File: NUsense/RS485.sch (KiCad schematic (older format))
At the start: 7 parts, among them J1101 MOLEX22-03-5045, U1101 MAX3443ECSA+

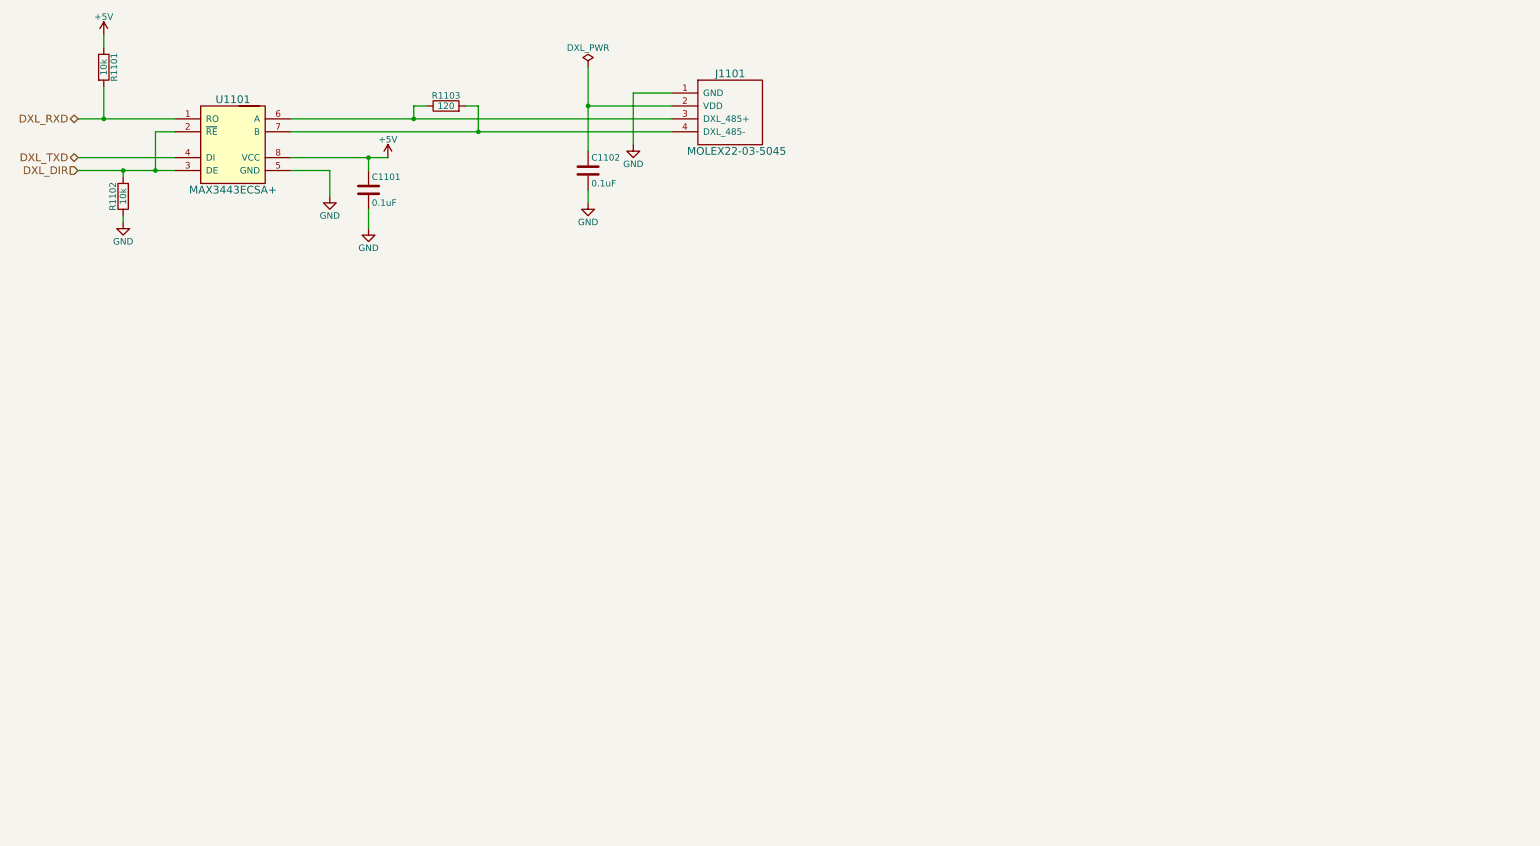
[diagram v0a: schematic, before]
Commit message: Cleans up some minor things
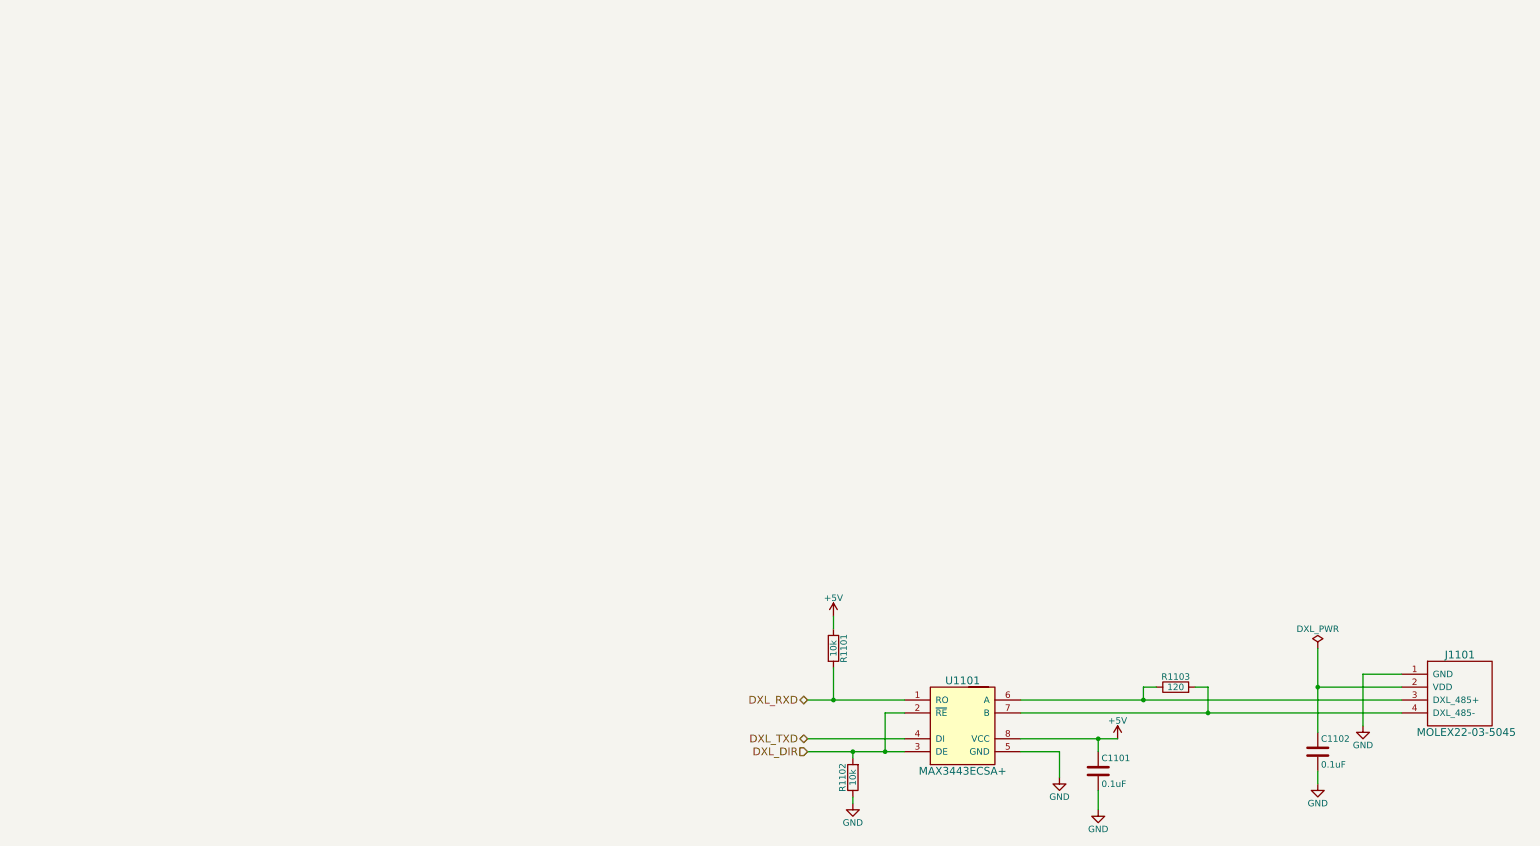
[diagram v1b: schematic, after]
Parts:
- renumbered C1101 to C501, C1102 to C502, J1101 to J501, R1101 to R501, R1102 to R502, R1103 to R503, U1101 to U501
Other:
- moved on the sheet: C1101, C1102, J1101, R1101, R1102, R1103, U1101
